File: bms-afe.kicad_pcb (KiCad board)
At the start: 2 copper layers, 45 x 58.5 mm, 121 parts, among them J1 CONN HEADER VERT 7POS 2.5MM, J2 CONN HEADER VERT 2POS 1.5MM, J3 CONN HEADER VERT 2POS 1.5MM, J4 CONN HEADER VERT 6POS 1.5MM, T1 PULSE XFMR 15UH 1 OHM FOR PLC, U1 TLE9012DQUXUMA1

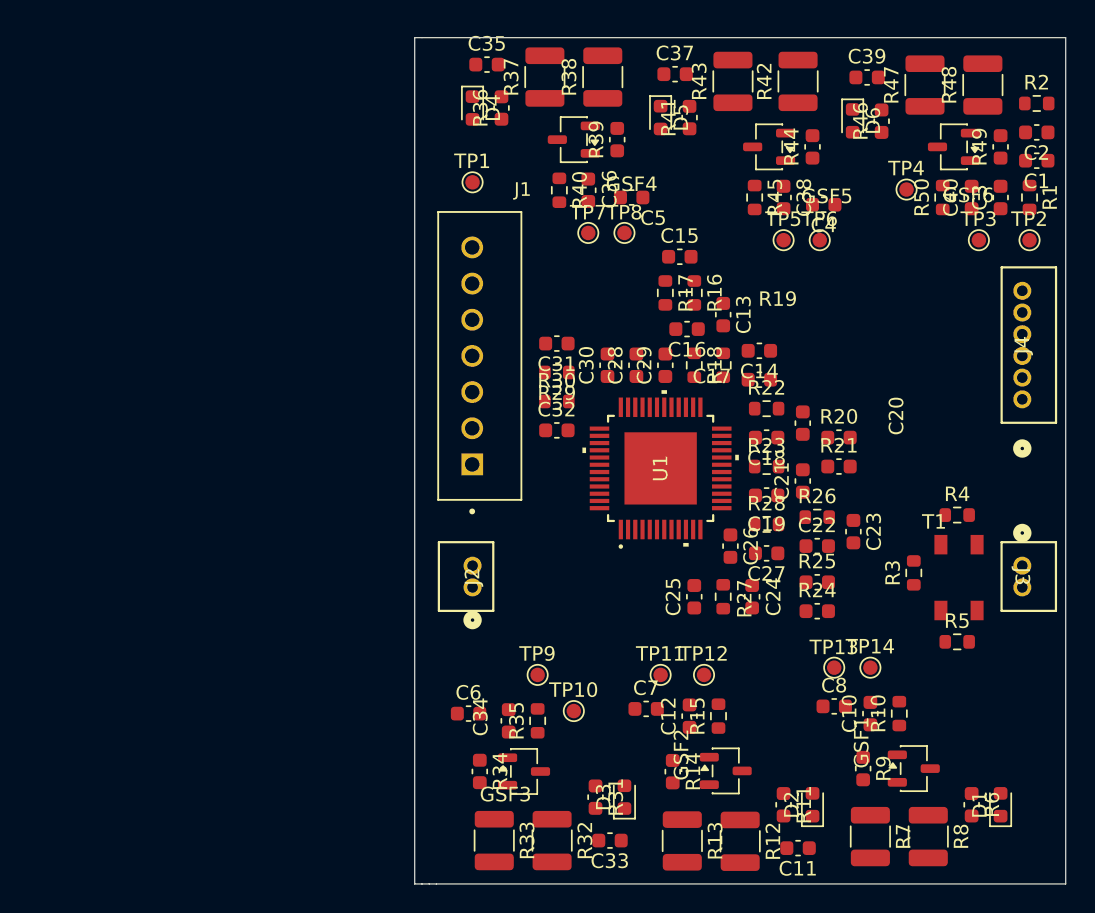
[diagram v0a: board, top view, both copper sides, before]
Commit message: first layout
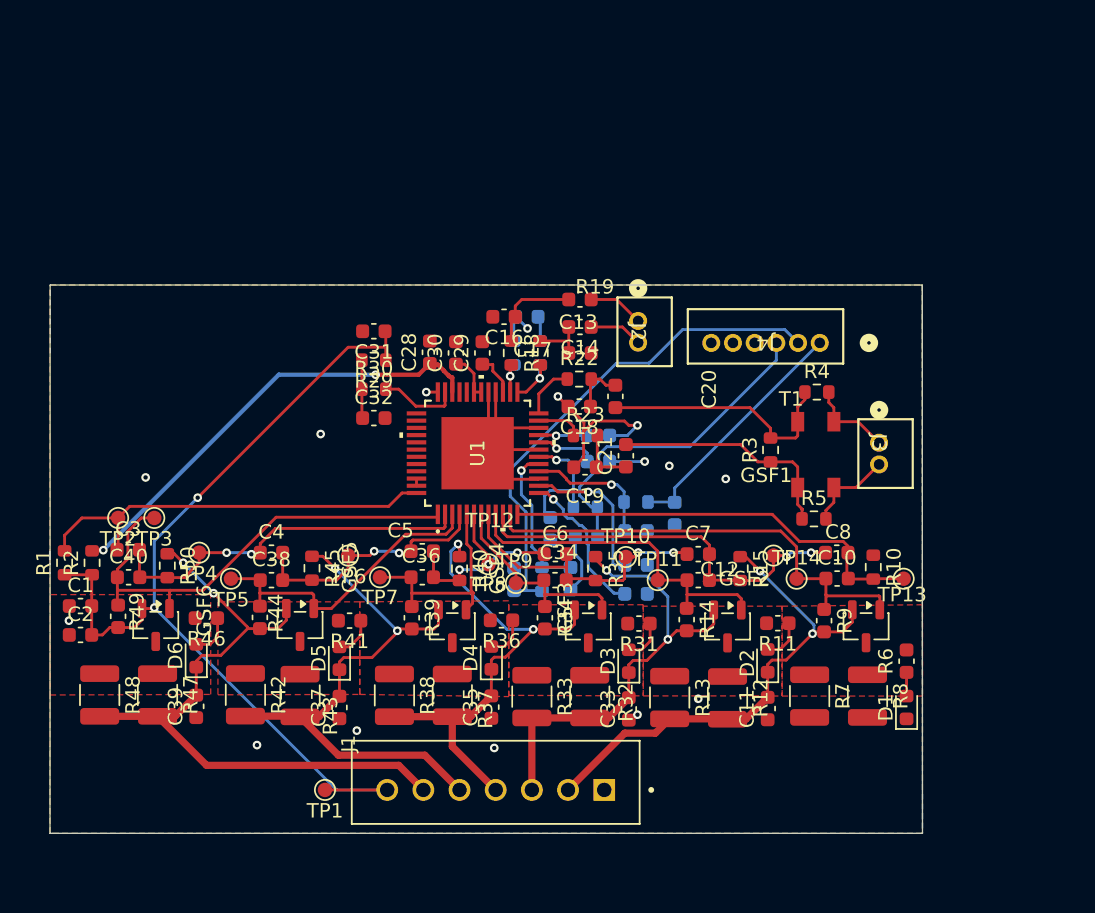
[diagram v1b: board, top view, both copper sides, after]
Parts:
- C15, C22, C23, C24, C25, C26, C27, R16, R17, R20, R21, R24, R25, R26, R27, R28: moved to B.Cu
- moved C2 74.7 mm to (67.4, 116.8), turned to 0 degrees
- moved R48 74.2 mm to (68.7, 120.9), turned to -90 degrees
- moved C1 72.9 mm to (67.4, 114.8), turned to 0 degrees
- moved R2 72.6 mm to (68.2, 111.8), turned to 90 degrees
- moved R1 71.3 mm to (66.3, 111.8), turned to 90 degrees
- moved R49 69.1 mm to (70.0, 115.5), turned to -90 degrees
- moved R47 67.8 mm to (72.7, 120.9), turned to -90 degrees
- moved TP2 65.9 mm to (70.0, 108.7), turned to 180 degrees
- moved C3 65.0 mm to (70.7, 110.9), turned to 0 degrees
- moved GSF6 64.3 mm to (72.6, 116.1), turned to -90 degrees
- moved C40 63.9 mm to (70.7, 112.8), turned to 0 degrees
- moved C39 63.6 mm to (75.4, 121.7), turned to 90 degrees
- moved TP3 60.1 mm to (72.5, 108.7), turned to 180 degrees
- moved R50 59.3 mm to (73.4, 112.0), turned to -90 degrees
- moved D6 58.5 mm to (75.4, 118.2), turned to 90 degrees
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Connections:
- C19 pad 2: BAT_GND -> BATGND
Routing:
- net /AFEIC/U12P: track 0.00 -> 65.4 mm, vias 0 -> 2
- net /CellBalance4/Battery_Pos: track 0.00 -> 46.1 mm, vias 0 -> 2
- net BATGND: track 0.00 -> 45.6 mm, vias 0 -> 14
- net /CellBalance3/Battery_Pos: track 0.00 -> 39.6 mm, vias 0 -> 2
- net /AFEIC/TMP1: track 0.00 -> 35.1 mm
- net /CellBalance/Battery_Pos: track 0.00 -> 34.4 mm, vias 0 -> 2
- net /CellBalance2/Battery_Pos: track 0.00 -> 34.3 mm, vias 0 -> 2
- net /AFEIC/G5: track 0.00 -> 33.2 mm
- net /AFEIC/G0: track 0.00 -> 32.4 mm
- net /CellBalance1/Battery_Pos: track 0.00 -> 31.7 mm, vias 0 -> 2
- net VBLK: track 0.00 -> 31.7 mm, vias 0 -> 2
- net /AFEIC/U0: track 0.00 -> 29.9 mm
- net /AFEIC/U6: track 0.00 -> 28.8 mm
- net /AFEIC/U1: track 0.00 -> 28.4 mm, vias 0 -> 2
- net /AFEIC/U5: track 0.00 -> 26.3 mm, vias 0 -> 2
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- added copper zone on B.Cu, net BATGND
- added copper zone on F.Cu, net BATGND
- added copper zone on F.Cu, net Net-(GSF1-D)
- added copper zone on F.Cu, net Net-(GSF2-D)
- added copper zone on F.Cu, net Net-(GSF3-D)
- added copper zone on F.Cu, net Net-(GSF4-D)
- added copper zone on F.Cu, net Net-(GSF5-D)
- added copper zone on F.Cu, net Net-(GSF6-D)
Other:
- board size 45 x 58.5 mm -> 60.3 x 37.9 mm

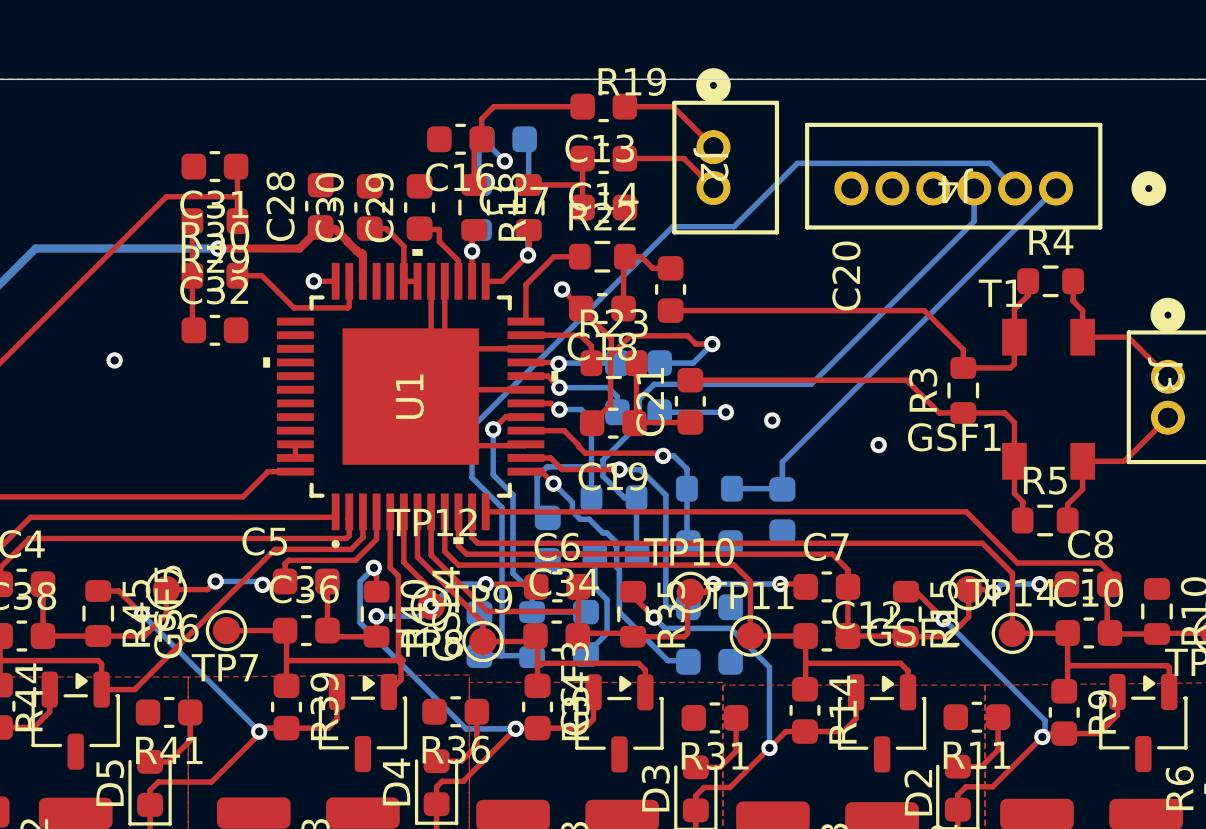
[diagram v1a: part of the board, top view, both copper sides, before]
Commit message: fixed minor layout changes
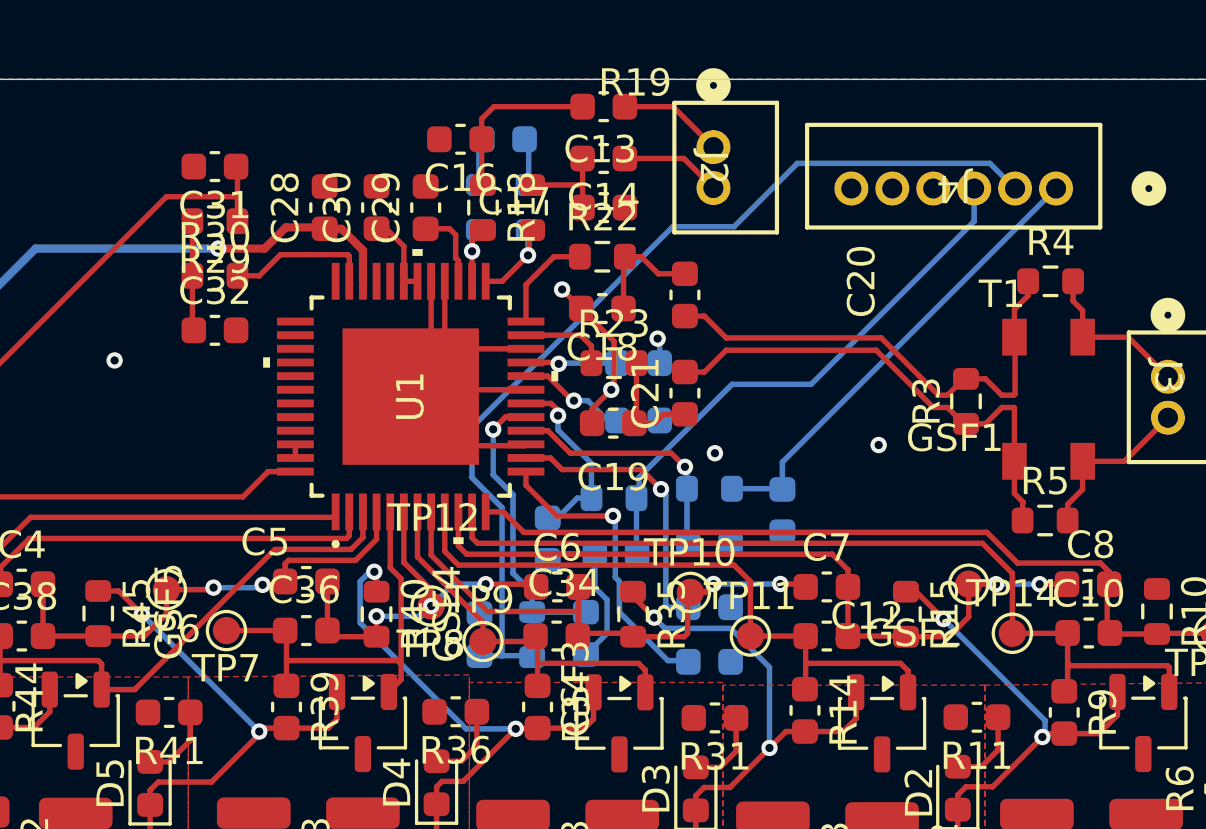
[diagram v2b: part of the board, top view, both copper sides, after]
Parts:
- moved C20 0.56 mm to (104.9, 100.5)
- moved R3 0.41 mm to (115.2, 104.4)
- moved C21 0.36 mm to (104.9, 104.1)
- moved R18 0.32 mm to (97.5, 97.3)
- moved R21 0.30 mm to (103.2, 105.1)
- moved C30 0.25 mm to (93.6, 97.3)
- moved C29 0.22 mm to (95.4, 97.3)
- moved TP12 0.20 mm to (115.3, 111.1)
- moved C28 0.16 mm to (91.7, 97.3)
- moved R19 0.12 mm to (99.3, 97.3)
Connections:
- net /AFEIC/IFH_H renamed /AFEIC/IFH_P
- net /AFEIC/IFH_H_Filt renamed /AFEIC/IFH_Filt_P
- net /AFEIC/IFH_L renamed /AFEIC/IFH_N
- net /AFEIC/IFH_L_Filt renamed /AFEIC/IFH_Filt_N
- net /AFEIC/IFL_H renamed /AFEIC/IFL_P
- net /AFEIC/IFL_L renamed /AFEIC/IFL_N
- R22 pad 1: /AFEIC/IFL_H_Filt -> /AFEIC/IFL_Filt_P
- R23 pad 1: /AFEIC/IFL_L_Filt -> /AFEIC/IFL_Filt_N
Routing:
- net BATGND: track 45.6 -> 37.0 mm, vias 14 -> 13
- net /AFEIC/TMP0: track 23.2 -> 20.2 mm
- net Net-(U1A-TMP0): track 9.33 -> 6.94 mm
- net /AFEIC/IFL_N: track 16.3 -> 18.0 mm
- net Net-(U1A-TMP4): track 10.5 -> 11.6 mm
- net Net-(C15-Pad1): track 2.88 -> 1.75 mm, vias 1 -> 0
- net /AFEIC/IFL_P: track 17.2 -> 18.2 mm
- net Net-(C18-Pad1): track 3.77 -> 4.38 mm
